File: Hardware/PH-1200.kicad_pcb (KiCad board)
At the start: 2 copper layers, 120 x 80 mm, 69 parts, among them J1 SW_ONOFF, J2 SW_INV, J3 SENSOR LÍNEA, J4 RESET, J5 USB_B, J6 12V, J7 GND, K1 SRD-05VDC-SL-C, K2 SRD-05VDC-SL-C, Q1 MMBT3904, Q2 MMBT3904, Q3 MMBT3904, Q4 MMBT3904, Q6 MMBT3906, Q7 MMBT3906, SW1 SW_ENC, U1 TPS562207S, U2 4N28X, U3 6N137S, U4 6N137S, U5 CP2102N-A02-GQFN24, U6 SRV05-4

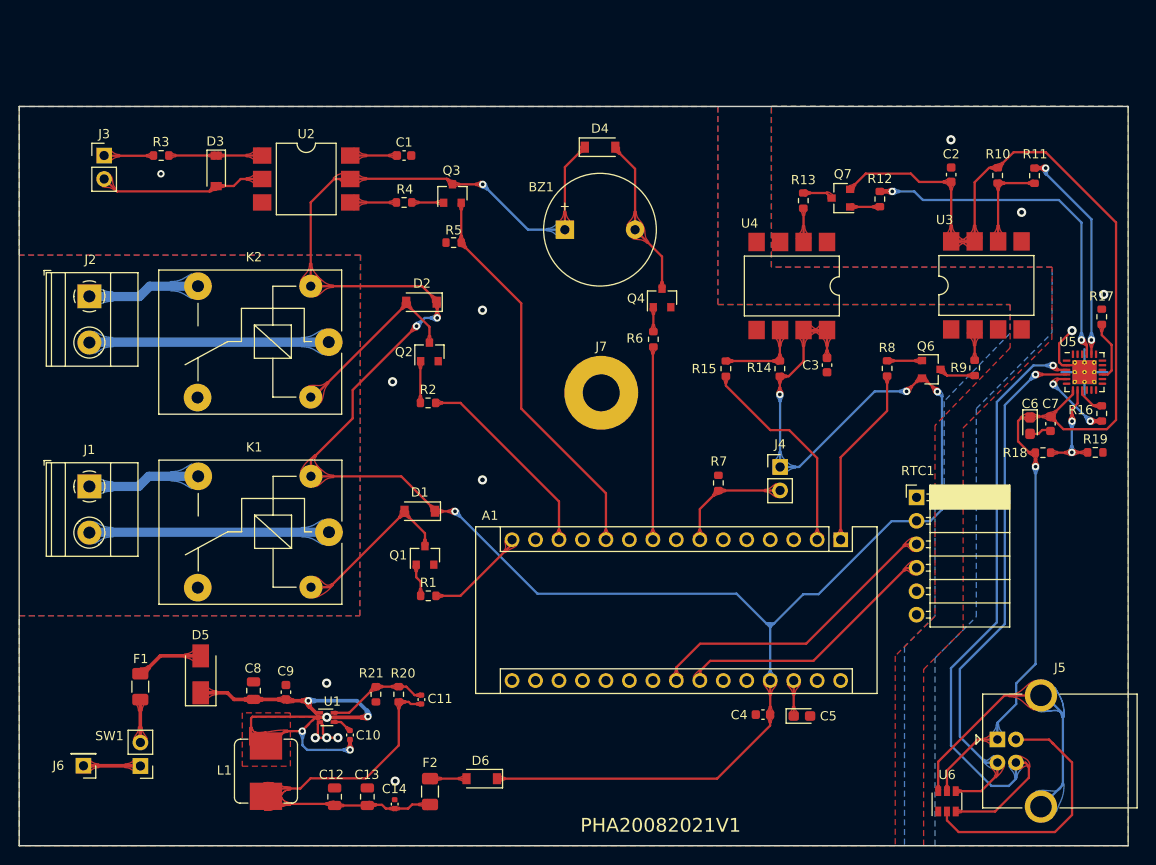
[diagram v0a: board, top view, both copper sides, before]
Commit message: Update KiCad files
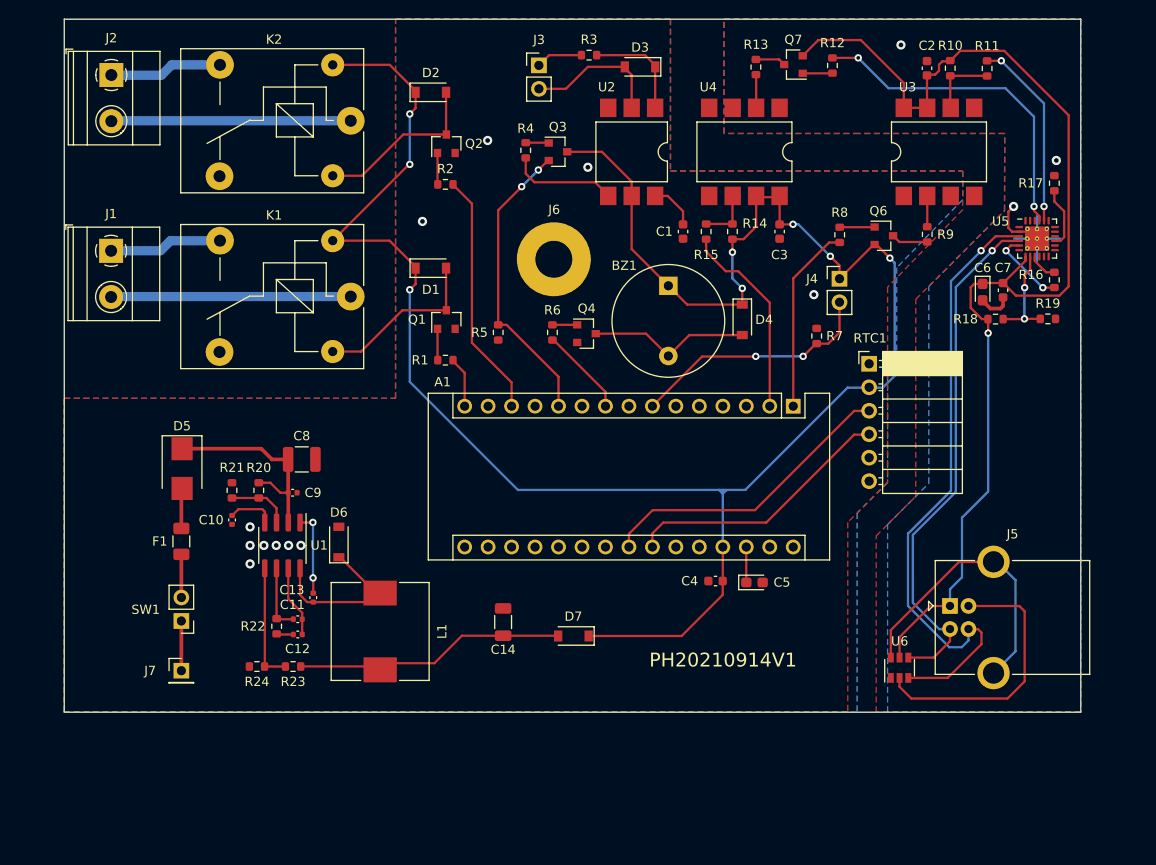
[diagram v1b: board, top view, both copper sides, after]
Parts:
- removed F2: 0.25 A, Fuse:Fuse_1206_3216Metric
- added D7: B5817W, Diode_SMD:D_SOD-123, F.Cu at (135.1, 126.8)
- added R22: 5.49K, Resistor_SMD:R_0603_1608Metric, F.Cu at (103.0, 125.8)
- added R23: 10.2K, Resistor_SMD:R_0603_1608Metric, F.Cu at (104.8, 130.1)
- added R24: 1.58K, Resistor_SMD:R_0603_1608Metric, F.Cu at (100.8, 130.1)
- C10: value 100nF -> 8.2nF
- C11: value 22pF -> 10pF
- C12: value 22uF -> 6.8nF; footprint Capacitor_SMD:C_0805_2012Metric -> Capacitor_SMD:C_0402_1005Metric
- C13: value 22uF -> 100nF; footprint Capacitor_SMD:C_0805_2012Metric -> Capacitor_SMD:C_0402_1005Metric
- C14: value 100nF -> 10uF; footprint Capacitor_SMD:C_0402_1005Metric -> Capacitor_SMD:C_1206_3216Metric
- C8: value 10uF -> 22uF; footprint Capacitor_SMD:C_0805_2012Metric -> Capacitor_SMD:C_1210_3225Metric
- C9: footprint Capacitor_SMD:C_0603_1608Metric -> Capacitor_SMD:C_0402_1005Metric
- D5: footprint Diode_SMD:D_SMA -> Diode_SMD:D_SMB
- F1: value 0.5 A -> 0.75 A
- J6: value 12V -> GND; footprint Connector_PinHeader_2.54mm:PinHeader_1x01_P2.54mm_Vertical -> MountingHole:MountingHole_4mm_Pad
- J7: value GND -> 12V; footprint MountingHole:MountingHole_4mm_Pad -> Connector_PinHeader_2.54mm:PinHeader_1x01_P2.54mm_Vertical
- L1: value 4.7uH -> 47uH; footprint Inductor_SMD:L_Bourns_SRP7028A_7.3x6.6mm -> Inductor_SMD:L_10.4x10.4_H4.8
- R20: value 64.9K -> 169K
- R21: value 10K -> 42.2K
- U1: value TPS562207S -> TPS54231DR; footprint Package_TO_SOT_SMD:SOT-563 -> Package_SO:SOIC-8_3.9x4.9mm_P1.27mm
- moved J6 74.8 mm to (133.0, 86.1)
- moved J7 54.5 mm to (92.7, 130.6)
- moved J3 48.1 mm to (131.4, 65.1)
- moved R3 47.6 mm to (136.8, 64.0)
- moved D3 47.2 mm to (142.3, 65.2), turned to 180 degrees
- moved U2 35.3 mm to (141.4, 74.4), turned to 270 degrees
- moved C1 31.3 mm to (147.0, 83.1), turned to 270 degrees
- moved D6 29.9 mm to (109.7, 116.7), turned to 90 degrees
- moved R21 27.0 mm to (98.1, 111.1), turned to 90 degrees
- moved R20 26.8 mm to (101.0, 111.1), turned to 270 degrees
- moved C10 26.5 mm to (98.1, 114.3)
- moved D1 26.3 mm to (119.7, 87.0), turned to 0 degrees
- moved Q1 25.6 mm to (121.3, 92.6)
- moved J1 25.6 mm to (85.1, 85.1)
- moved K1 25.6 mm to (111.0, 90.1)
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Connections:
- C10 pad 2: Net-(C10-Pad2) -> GND
- C11 pad 2: Net-(C11-Pad2) -> GND
- C12 pad 1: Net-(C11-Pad1) -> Net-(C12-Pad1)
- C13 pad 1: Net-(C11-Pad1) -> Net-(C13-Pad1)
- C13 pad 2: GND -> Net-(C13-Pad2)
- C14 pad 1: Net-(C11-Pad1) -> Net-(C14-Pad1)
- D6 pad 1: +5V -> Net-(C13-Pad1)
- D6 pad 2: Net-(D6-Pad2) -> GND
- J6 pad 1: Net-(J6-Pad1) -> GND
- J7 pad 1: GND -> Net-(J7-Pad1)
- L1 pad 1: Net-(C10-Pad2) -> Net-(C13-Pad1)
- L1 pad 2: Net-(C11-Pad1) -> Net-(C14-Pad1)
- R20 pad 1: Net-(C11-Pad1) -> Net-(C8-Pad1)
- R20 pad 2: Net-(C11-Pad2) -> Net-(R20-Pad2)
- R21 pad 1: Net-(C11-Pad2) -> Net-(R20-Pad2)
- SW1 pad 1: Net-(J6-Pad1) -> Net-(J7-Pad1)
- U1 pad 1: Net-(C8-Pad1) -> Net-(C13-Pad2)
- U1 pad 2: Net-(C10-Pad2) -> Net-(C8-Pad1)
- U1 pad 3: GND -> Net-(R20-Pad2)
- U1 pad 5: Net-(C8-Pad1) -> Net-(R23-Pad2)
- U1 pad 6: Net-(C11-Pad2) -> Net-(C11-Pad1)
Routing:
- net +5V: track 271.2 -> 226.0 mm, vias 7 -> 8
- net Net-(C11-Pad1): track 42.3 -> 7.29 mm
- net Net-(C14-Pad1): track 0.00 -> 32.4 mm
- net Net-(C10-Pad2): track 28.1 -> 0.00 mm, vias 2 -> 0
- net Net-(C13-Pad1): track 0.00 -> 18.5 mm
- net RESET: track 13.3 -> 26.9 mm, vias 0 -> 2
- net Net-(R23-Pad2): track 0.00 -> 12.9 mm
- net BUZZER: track 21.4 -> 9.61 mm
- net Net-(C11-Pad2): track 11.0 -> 0.00 mm
- net VLINEA: track 43.3 -> 32.3 mm, vias 0 -> 2
- net Net-(C13-Pad2): track 0.00 -> 9.09 mm, vias 0 -> 2
- net VBUS: track 131.3 -> 123.0 mm
- net Net-(R20-Pad2): track 0.00 -> 6.84 mm
- net Net-(R4-Pad2): track 5.00 -> 11.7 mm
- net Net-(J6-Pad1): track 6.17 -> 0.00 mm
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- removed copper zone on F.Cu, net Net-(C10-Pad2)
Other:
- board size 120 x 80 mm -> 110 x 75 mm
- board text added: "PH20210914V1"
- board text removed: "PHA20082021V1"
